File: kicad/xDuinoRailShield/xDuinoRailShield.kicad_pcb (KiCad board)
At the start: 2 copper layers, 59.7 x 21.9 mm, 19 parts, among them J105 21mtc_mrkl, Q501 S8050, Q502 S8550, Q503 S8550, Q504 S8050, U601 MOUDLE-SEEEDUINO-XIAO-ESP32C3, U801 L78L05_SOT89, U901 ULN2003A, U902 DRV8872DDA

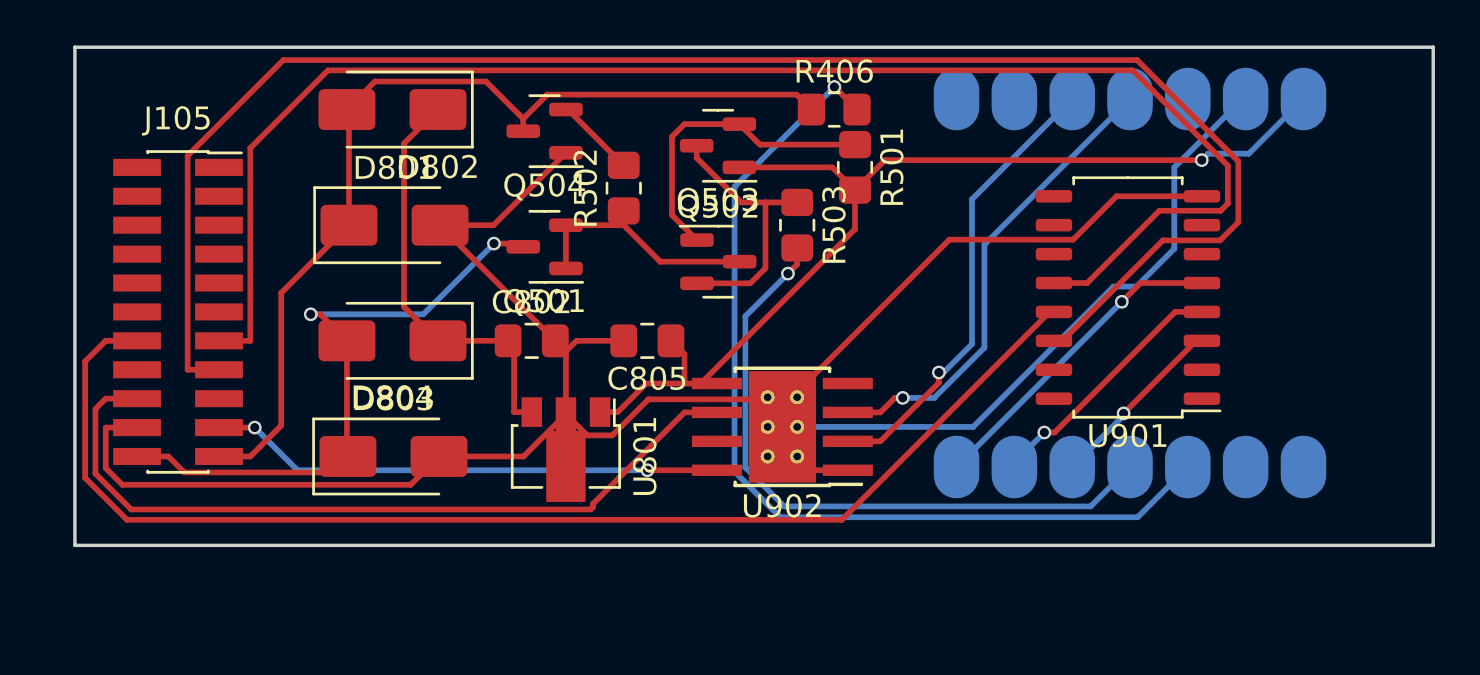
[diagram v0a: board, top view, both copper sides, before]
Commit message: A lot of fixes
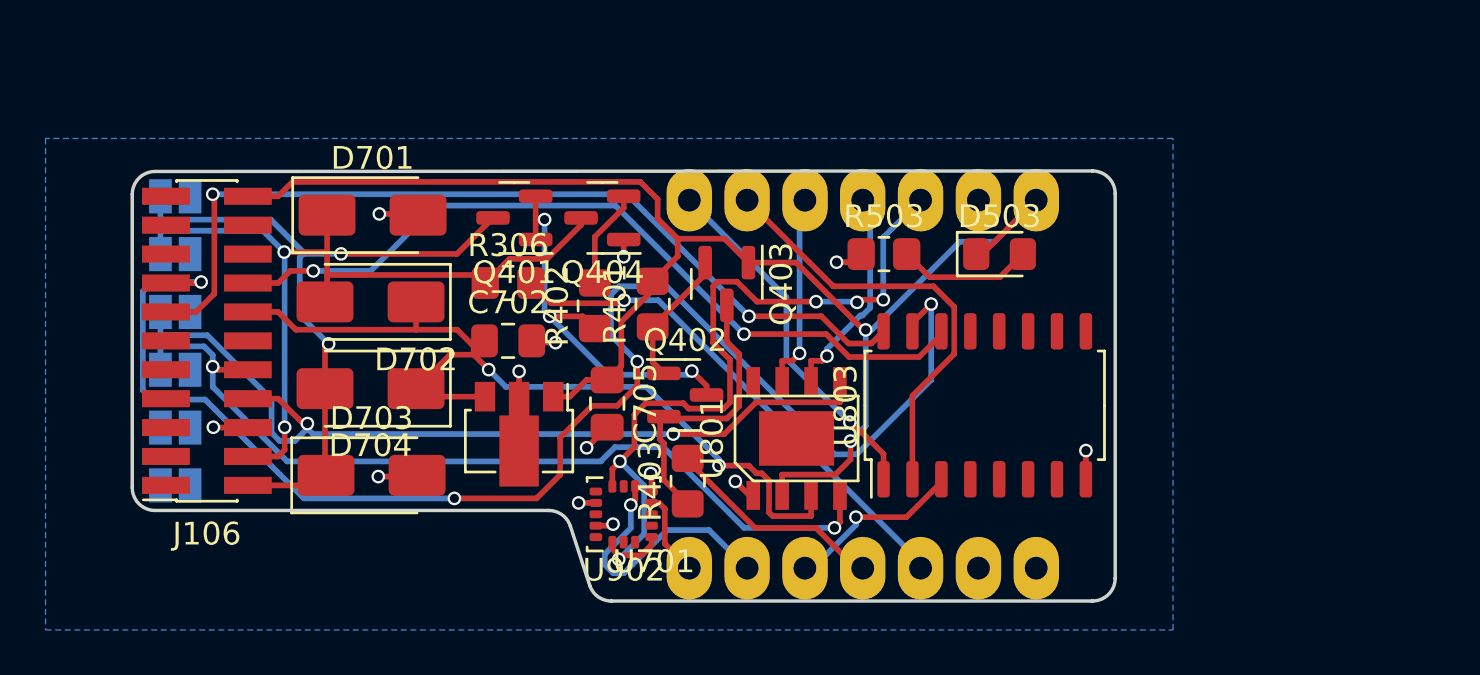
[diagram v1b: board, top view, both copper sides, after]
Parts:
- removed J105: 21mtc_mrkl, Connector_PinSocket_1.27mm:PinSocket_2x11_P1.27mm_Vertical_SMD
- added D503: LED, LED_SMD:LED_0805_2012Metric_Pad1.15x1.40mm_HandSolder, F.Cu at (162.2, 70.8)
- added J106: 21mtc_mrkl, Connector_PinSocket_1.27mm:PinSocket_2x11_P1.27mm_Vertical_SMD, F.Cu at (127.4, 74.6)
- added JP101: SolderJumper_2_Bridged, Jumper:SolderJumper-2_P1.3mm_Bridged_Pad1.0x1.5mm, B.Cu at (126.0, 70.8)
- added JP102: SolderJumper_2_Bridged, Jumper:SolderJumper-2_P1.3mm_Bridged_Pad1.0x1.5mm, B.Cu at (126.0, 68.2)
- added JP103: SolderJumper_2_Bridged, Jumper:SolderJumper-2_P1.3mm_Bridged_Pad1.0x1.5mm, B.Cu at (126.0, 75.9)
- added JP104: SolderJumper_2_Bridged, Jumper:SolderJumper-2_P1.3mm_Bridged_Pad1.0x1.5mm, B.Cu at (126.0, 73.3)
- added JP105: SolderJumper_2_Bridged, Jumper:SolderJumper-2_P1.3mm_Bridged_Pad1.0x1.5mm, B.Cu at (126.0, 78.4)
- added JP106: SolderJumper_2_Bridged, Jumper:SolderJumper-2_P1.3mm_Bridged_Pad1.0x1.5mm, B.Cu at (126.0, 81.0)
- added R503: 1k, Resistor_SMD:R_0805_2012Metric_Pad1.20x1.40mm_HandSolder, F.Cu at (157.2, 70.8)
- added U801: BDR6133, BDR6133:BDR6133, F.Cu at (153.3, 78.9)
- U902: value DRV8872DDA -> LIS3DH; footprint Package_SO:Texas_HTSOP-8-1EP_3.9x4.9mm_P1.27mm_EP2.95x4.9mm_Mask2.4x3.1mm_ThermalVias -> Package_LGA:LGA-16_3x3mm_P0.5mm_LayoutBorder3x5y
- moved R306 16.2 mm to (140.6, 72.1)
- moved U501 12.6 mm to (145.7, 85.4)
- moved R403 12.2 mm to (148.5, 80.8), turned to 90 degrees
- moved R401 10.7 mm to (147.0, 73.0), turned to 90 degrees
- moved D702 8.50 mm to (134.6, 72.9)
- moved U902 7.96 mm to (145.7, 82.2)
- moved U803 7.88 mm to (161.6, 77.4), turned to 90 degrees
- moved Q403 6.08 mm to (150.2, 72.1), turned to -90 degrees
- moved Q402 6.03 mm to (148.4, 77.0)
- moved R402 5.32 mm to (144.4, 73.1)
- moved Q404 4.58 mm to (144.8, 69.2)
- moved C705 3.27 mm to (145.0, 77.4), turned to -90 degrees
- moved D704 2.31 mm to (134.6, 76.7)
- moved U701 2.17 mm to (141.1, 79.0)
- moved Q401 1.84 mm to (140.9, 69.2)
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- renumbered C802 to C702, C805 to C705, D801 to D701, D802 to D702, D803 to D703, D804 to D704, Q501 to Q401, Q502 to Q402, Q503 to Q403, Q504 to Q404, R406 to R306, R501 to R401, R502 to R402, R503 to R403, U601 to U501, U801 to U701, U901 to U803
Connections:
- net /AUDIO renamed /MCU Carrier Board/EMF_MOTOR0
- net ACDC_SIGNAL renamed /MCU Carrier Board/EMF_MOTOR1
- net Net-(Q501-B) renamed /Railcom-Feedback/RC_SIGNAL
- net Net-(Q502-B) renamed /Railcom-Feedback/RC_FB_IN
- net Net-(Q502-E) renamed /Railcom-Feedback/RC_CURR
- net Net-(Q504-B) renamed /Railcom-Feedback/RC_ON_OFF
- U501 pad 12: unconnected-(U601-3V3-Pad12) -> +3V3
- U501 pad 6: /AUX2 -> /MCU Carrier Board/I2C1
- U501 pad 7: /AUX3 -> /MCU Carrier Board/I2C0
- U501 pad 8: /MCU Carrier Board/F0.BACKWARD -> /MCU Carrier Board/FUNC0
- U501 pad 9: /MCU Carrier Board/F0.FOREWARD -> /MCU Carrier Board/FUNC1
- U803 pad 1: /Motor and Power drivers/F00 -> /MCU Carrier Board/FUNC0
- U803 pad 10: /Motor and Power drivers/AMP_AUX5 -> unconnected-(U803-O7-Pad10)
- U803 pad 11: /Motor and Power drivers/AMP_AUX4 -> unconnected-(U803-O6-Pad11)
- U803 pad 12: AMP_AUX3 -> unconnected-(U803-O5-Pad12)
- U803 pad 13: AMP_AUX2 -> unconnected-(U803-O4-Pad13)
- U803 pad 14: AMP_AUX1 -> /Connectors 21mtc / PluXX / NEMA/AMP_AUX1
- U803 pad 15: /Motor and Power drivers/AMP_F01 -> /Connectors 21mtc / PluXX / NEMA/AMP_FUNC1
- U803 pad 16: /Motor and Power drivers/AMP_F00 -> /Connectors 21mtc / PluXX / NEMA/AMP_FUNC0
- U803 pad 2: /Motor and Power drivers/F01 -> /MCU Carrier Board/FUNC1
- U803 pad 4: /AUX2 -> unconnected-(U803-I4-Pad4)
- U803 pad 5: /AUX3 -> unconnected-(U803-I5-Pad5)
- U803 pad 6: /AUX4 -> unconnected-(U803-I6-Pad6)
- U803 pad 7: /AUX5 -> unconnected-(U803-I7-Pad7)
- U902 pad 1: GND -> +3V3
- U902 pad 2: /MCU Carrier Board/MOTOR1 -> unconnected-(U902-NC-Pad2)
- U902 pad 3: /MCU Carrier Board/MOTOR0 -> unconnected-(U902-NC-Pad3)
- U902 pad 4: unconnected-(U902-nFAULT-Pad4) -> /MCU Carrier Board/I2C0
- U902 pad 5: +5V -> GND
- U902 pad 6: /Connectors 21mtc / PluXX / NEMA/AMP_MOTOR0 -> /MCU Carrier Board/I2C1
- U902 pad 8: /Connectors 21mtc / PluXX / NEMA/AMP_MOTOR1 -> +3V3
- U902 pad 9: GND -> unconnected-(U902-INT2-Pad9)
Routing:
- net GND: track 114.0 -> 15.2 mm, vias 0 -> 13
- net AMP_AUX1: track 73.5 -> 0.00 mm
- net AMP_AUX3: track 66.7 -> 0.00 mm
- net /Connectors 21mtc / PluXX / NEMA/AMP_FUNC1: track 0.00 -> 63.3 mm, vias 0 -> 4
- net AMP_AUX2: track 54.9 -> 0.00 mm
- net /Connectors 21mtc / PluXX / NEMA/AMP_FUNC0: track 0.00 -> 39.3 mm, vias 0 -> 2
- net /Connectors 21mtc / PluXX / NEMA/AMP_AUX1: track 0.00 -> 35.2 mm, vias 0 -> 2
- net +3V3: track 0.00 -> 34.7 mm, vias 0 -> 5
- net DCC_VIN: track 18.5 -> 38.7 mm, vias 0 -> 2
- net /MCU Carrier Board/FUNC1: track 0.00 -> 19.4 mm
- net DCC_MM: track 41.8 -> 22.6 mm
- net RAILCOM_DATA: track 28.9 -> 9.74 mm, vias 1 -> 0
- net +5V: track 45.9 -> 64.4 mm, vias 1 -> 2
- net /Connectors 21mtc / PluXX / NEMA/AMP_MOTOR1: track 22.7 -> 38.7 mm
- net /MCU Carrier Board/FUNC0: track 0.00 -> 15.8 mm, vias 0 -> 1
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- added copper zone on B.Cu, net GND
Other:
- board size 59.7 x 21.9 mm -> 43.2 x 18.9 mm
